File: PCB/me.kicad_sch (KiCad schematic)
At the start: 14 parts, among them M1 Motor_DC, Q1 AO3400A, SW1 SW_Push, SW2 SW_Push, SW3 SW_Push, SW4 SW_Push, SW5 SW_Push, SW6 SW_Push, U1 XIAO-RP2040-DIP

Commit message: uohewf
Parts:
- U1: footprint RF_Module:MCU_Seeed_ESP32C3 -> Seeed Studio XIAO Series Library:XIAO-RP2040-DIP
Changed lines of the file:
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@@
 			)
 		)
-		(property "Footprint" "RF_Module:MCU_Seeed_ESP32C3"
+		(property "Footprint" "Seeed Studio XIAO Series Library:XIAO-RP2040-DIP"
 			(at 114.808 98.298 0)
 			(effects

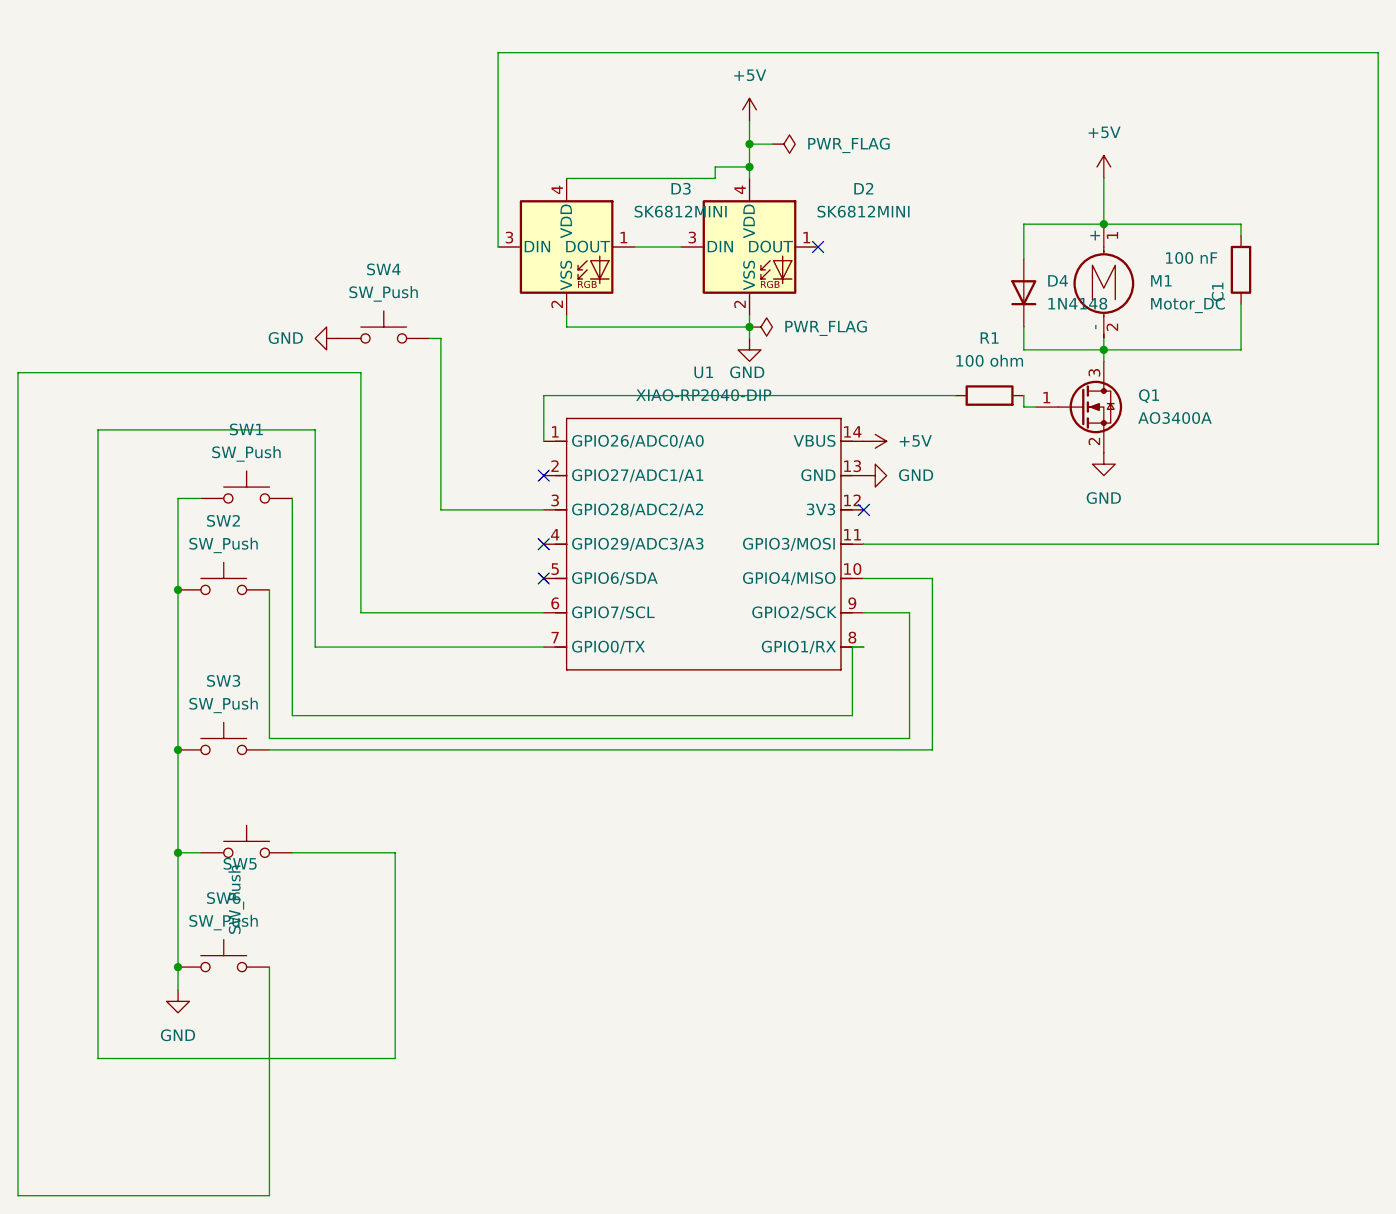
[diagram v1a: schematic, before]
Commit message: i hate this
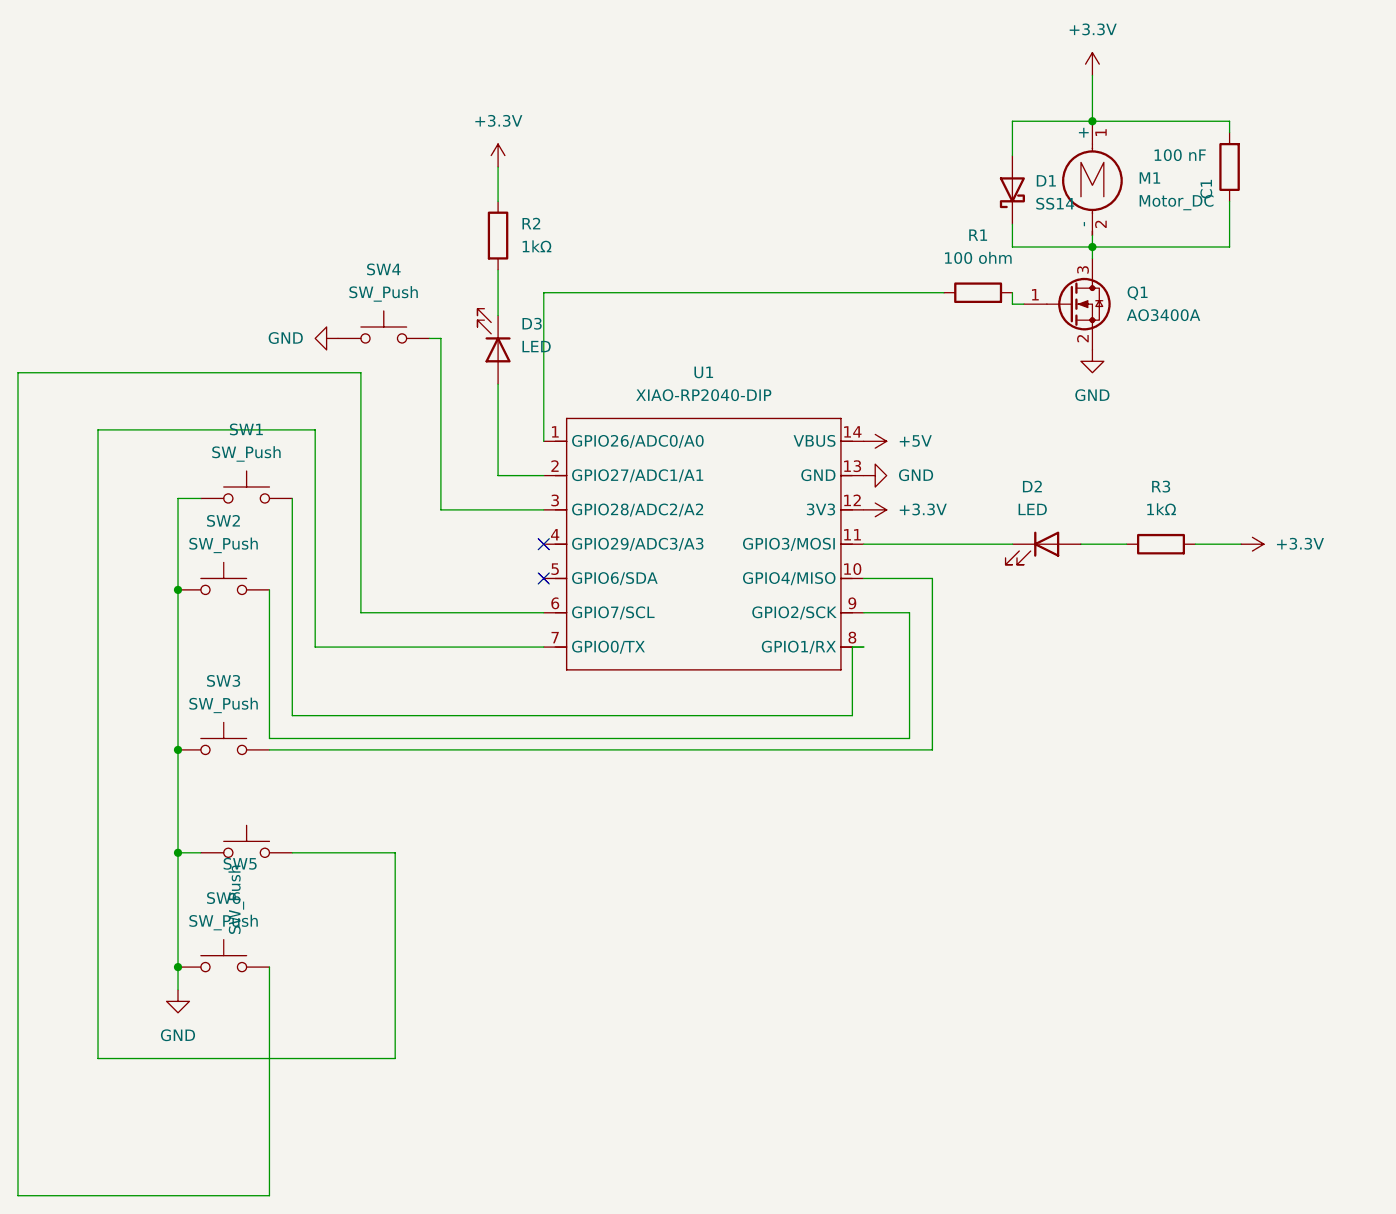
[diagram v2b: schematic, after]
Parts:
- removed D2, D3: SK6812MINI, LED_SMD:LED_SK6812MINI_PLCC4_3.5x3.5mm_P1.75mm, symbol LED:SK6812MINI
- removed D4: 1N4148, Diode_THT:D_DO-35_SOD27_P7.62mm_Horizontal, symbol Diode:1N4148
- added D1: SS14, Diode_SMD:D_SMA, symbol Diode:SS14
- added D2, D3: LED, LED_SMD:LED_0603_1608Metric, symbol Device:LED
- added R2, R3: 1kΩ, Resistor_SMD:R_0603_1608Metric, symbol Device:R
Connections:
- net +5V: no longer C1.2, M1.1 (+)
- net at U1.11 (GPIO3/MOSI): now also D2.1 (K)
- net +3.3V: now reaches U1.12 (3V3)
- net +3.3V: now also C1.2, M1.1 (+), D1.2 (A), R2.1, R3.2
- net at U1.2 (GPIO27/ADC1/A1): now also D3.2 (A)
- net at C1.1, M1.2 (-), Q1.3 (D): now also D1.1 (K)
- new net: D3.1 (K), R2.2
- new net: D2.2 (A), R3.1
- no-connect marks 5 -> 2
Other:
- moved on the sheet: C1, M1, Q1, R1
